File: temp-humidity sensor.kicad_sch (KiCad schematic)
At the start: 43 parts, among them J1 Conn_01x02, J2 USB_C_Receptacle_USB2.0_16P, SW1 SW_Push, SW2 SW_Push, SW3 SS-12D01-G040, U1 SHT4x, U2 ESP32-C6-WROOM-1, U3 BQ24074RGT, U4 USBLC6-2SC6, U5 TPS63031DSK

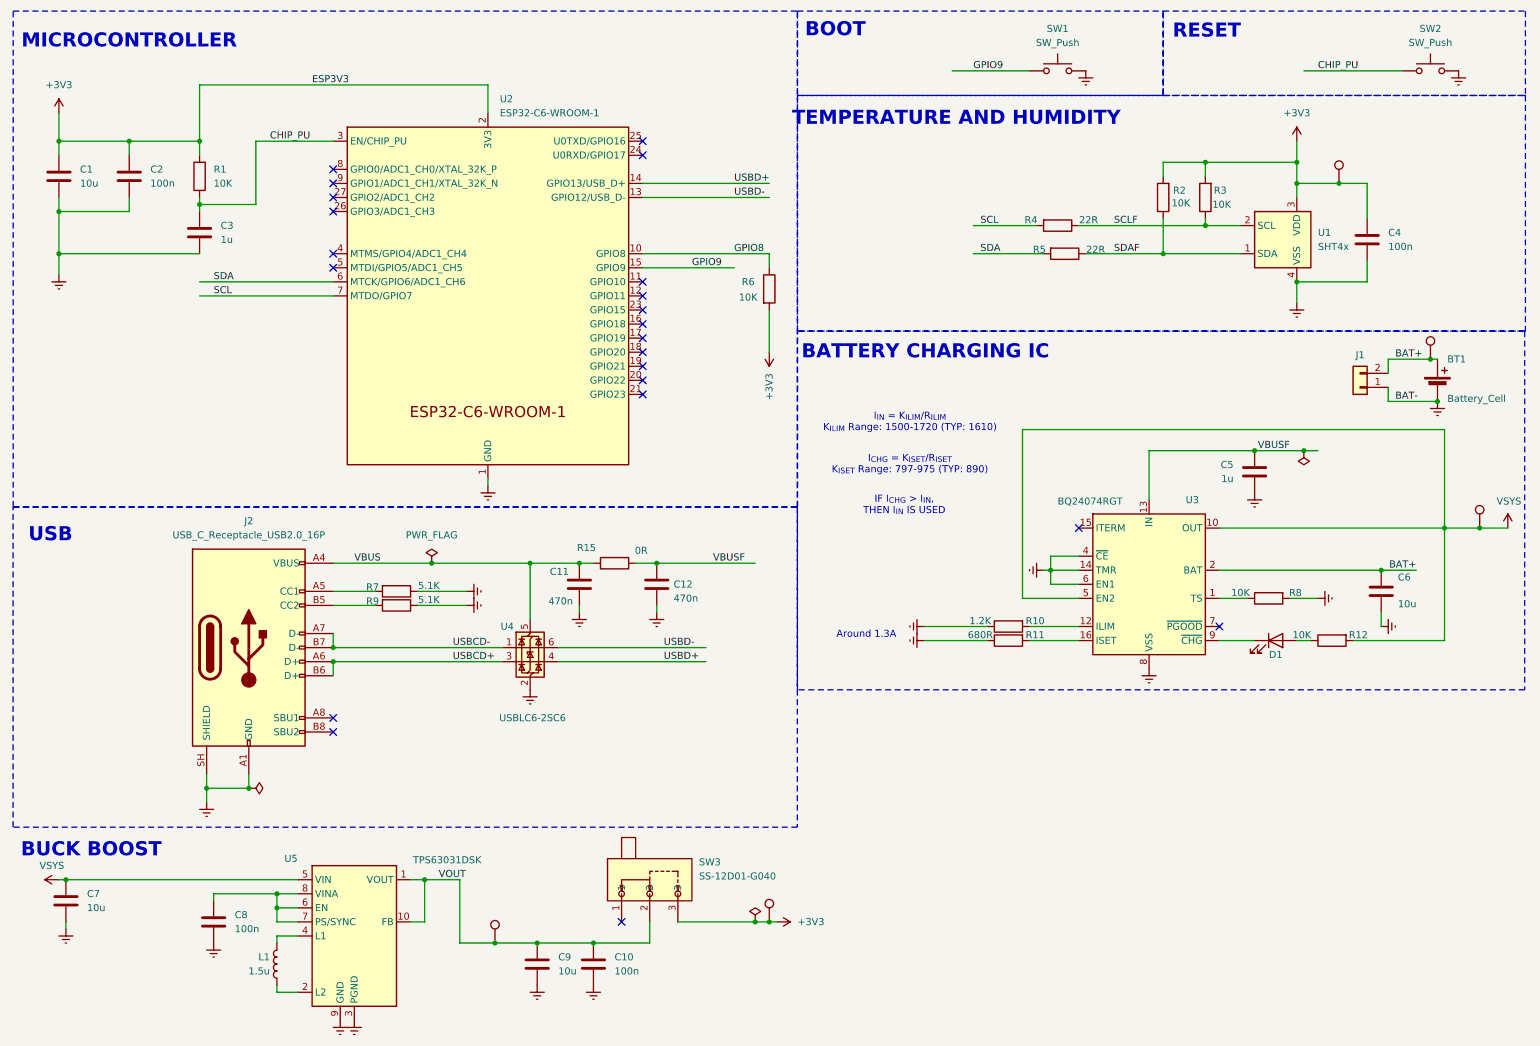
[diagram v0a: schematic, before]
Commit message: V3
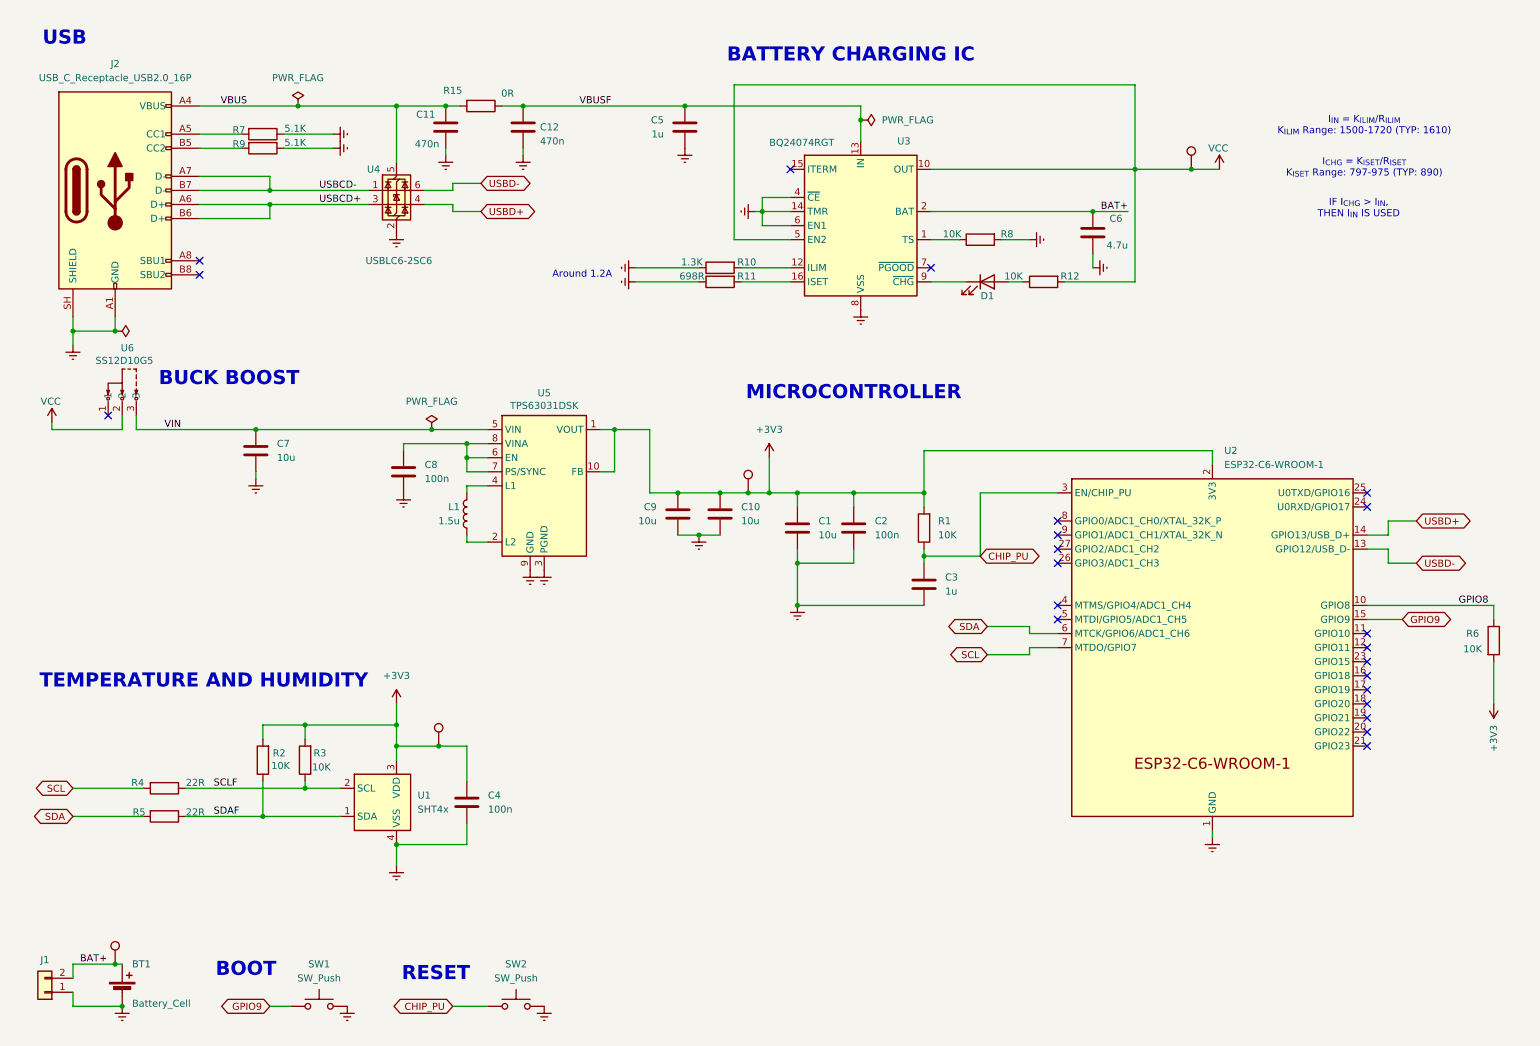
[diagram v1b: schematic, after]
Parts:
- removed SW3: SS-12D01-G040, easyeda2kicad:SW-TH_SS-12D01-GX, symbol LCSC:SS-12D01-G040
- removed TP6: TestPoint, TestPoint:TestPoint_Pad_D1.0mm, symbol Connector:TestPoint
- added U6: SS12D10G5, easyeda2kicad:SW-TH_SHOU-HAN_SS12D10G4, symbol easyeda2kicad:SS12D10G5
- C1, C7, C9: footprint Capacitor_SMD:C_0603_1608Metric -> Capacitor_SMD:C_0805_2012Metric; LCSC C19702 -> C5448891
- C10: value 100n -> 10u; footprint Capacitor_SMD:C_0603_1608Metric -> Capacitor_SMD:C_0805_2012Metric; LCSC C19702 -> C5448891
- C2: footprint Capacitor_SMD:C_0603_1608Metric -> Capacitor_SMD:C_0805_2012Metric; LCSC C77055 -> C111492
- C3: LCSC C59302 -> C106248
- C5: footprint Capacitor_SMD:C_0603_1608Metric -> Capacitor_SMD:C_0805_2012Metric; LCSC C59302 -> C91185
- C6: value 10u -> 4.7u; footprint Capacitor_SMD:C_0603_1608Metric -> Capacitor_SMD:C_0805_2012Metric; LCSC C19702 -> C354262
- R10: value 1.2K -> 1.3K; LCSC C2906976 -> C2906977
- R11: value 680R -> 698R; LCSC C23228 -> C7467401
- U2: footprint PCM_Espressif_1:ESP32-C6-WROOM-1 -> PCM_Espressif:ESP32-C6-WROOM-1
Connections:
- net VOUT is gone; now on net +3V3: C10.1, C9.1, TP4.1, U5.1 (VOUT), U5.10 (FB)
- net VSYS renamed VCC
- net VCC: now also U6.2; no longer C7.1, U5.5 (VIN)
- new net VIN: C7.1, U5.5 (VIN), U6.3
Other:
- note added: "Around 1.2A"
- note removed: "Around 1.3A"
- moved on the sheet: BT1, C1, C11, C12, C2, C3, C4, C5, C6, C7, C8, D1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
